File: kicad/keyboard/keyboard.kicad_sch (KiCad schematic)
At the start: 119 parts, among them SW1 SW_MX, SW10 SW_MX, SW11 SW_MX, SW12 SW_MX, SW13 SW_MX, SW14 SW_MX, SW15 SW_MX, SW16 SW_MX, SW17 SW_MX, SW18 SW_MX, SW19 SW_MX, SW2 SW_MX, SW20 SW_MX, SW21 SW_MX, SW22 SW_MX, SW23 SW_MX, SW24 SW_MX, SW25 SW_MX, SW26 SW_MX, SW27 SW_MX, SW28 SW_MX, SW29 SW_MX, SW3 SW_MX, SW30 SW_MX, SW31 SW_MX, SW32 SW_MX, SW33 SW_MX, SW34 SW_MX, SW35 SW_MX, SW36 SW_MX, SW37 SW_MX, SW38 SW_MX, SW39 SW_MX, SW4 SW_MX, SW40 SW_MX, SW41 SW_MX, SW42 SW_MX, SW43 SW_MX, SW44 SW_MX, SW45 SW_MX, SW46 SW_MX, SW47 SW_MX, SW48 SW_MX, SW49 SW_MX, SW5 SW_MX, SW50 SW_MX, SW51 SW_MX, SW52 SW_MX, SW53 SW_MX, SW54 SW_MX, SW55 SW_MX, SW56 SW_MX, SW57 SW_MX, SW58 SW_MX, SW59 SW_MX, SW6 SW_MX, SW7 SW_MX, SW8 SW_MX, SW9 SW_MX

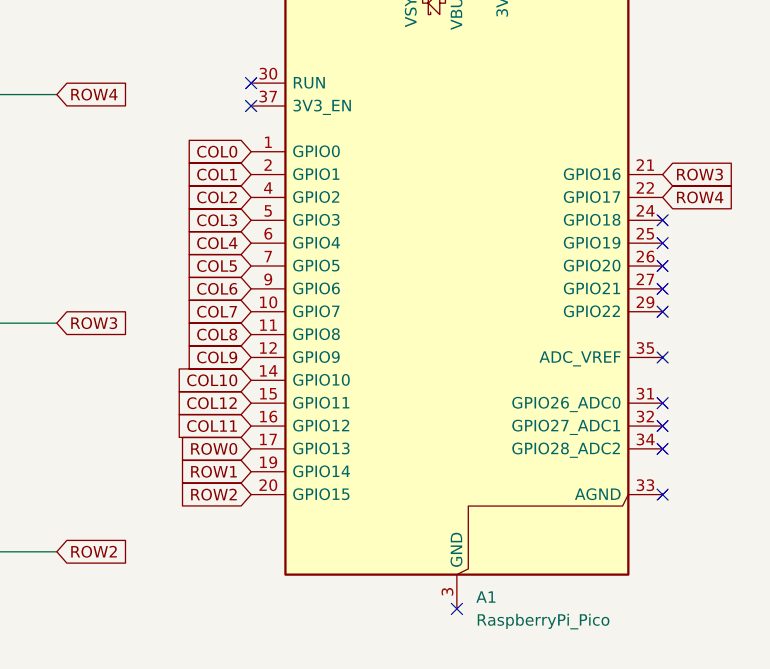
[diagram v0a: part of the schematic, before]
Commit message: Matrix traces
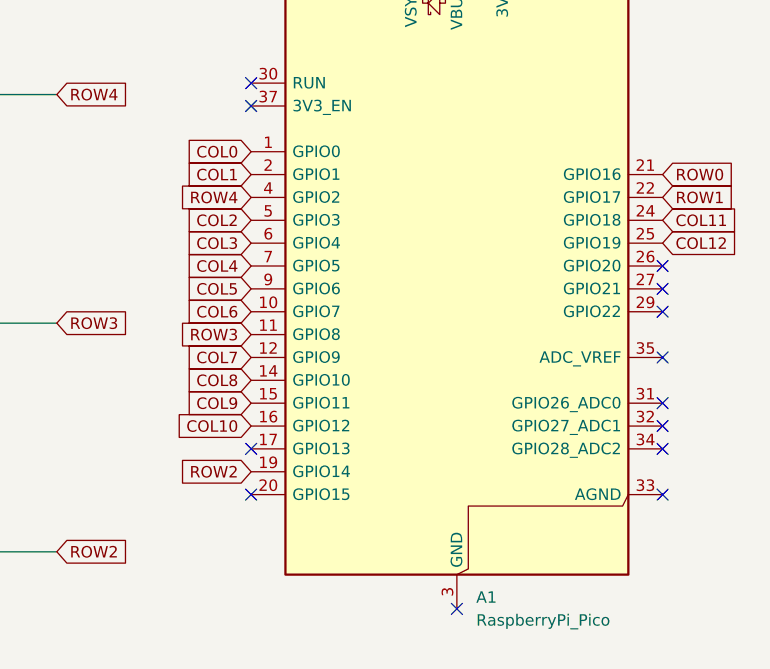
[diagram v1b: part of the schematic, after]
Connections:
- net COL10: now also A1.16 (GPIO12); no longer A1.14 (GPIO10)
- net COL11: now also A1.24 (GPIO18); no longer A1.16 (GPIO12)
- net COL12: now also A1.25 (GPIO19); no longer A1.15 (GPIO11)
- net COL2: now also A1.5 (GPIO3); no longer A1.4 (GPIO2)
- net COL3: now also A1.6 (GPIO4); no longer A1.5 (GPIO3)
- net COL4: now also A1.7 (GPIO5); no longer A1.6 (GPIO4)
- net COL5: now also A1.9 (GPIO6); no longer A1.7 (GPIO5)
- net COL6: now also A1.10 (GPIO7); no longer A1.9 (GPIO6)
- net COL7: now also A1.12 (GPIO9); no longer A1.10 (GPIO7)
- net COL8: now also A1.14 (GPIO10); no longer A1.11 (GPIO8)
- net COL9: now also A1.15 (GPIO11); no longer A1.12 (GPIO9)
- net ROW0: now also A1.21 (GPIO16); no longer A1.17 (GPIO13)
- net ROW1: now also A1.22 (GPIO17); no longer A1.19 (GPIO14)
- net ROW2: now also A1.19 (GPIO14); no longer A1.20 (GPIO15)
- net ROW3: now also A1.11 (GPIO8); no longer A1.21 (GPIO16)
- net ROW4: now also A1.4 (GPIO2); no longer A1.22 (GPIO17)
